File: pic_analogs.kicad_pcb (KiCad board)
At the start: 2 copper layers, 99.1 x 98.4 mm, 242 parts, among them J1 VFWD, J10 USB_B_Mini, J11 term_, J12 term_, J13 term_, J14 term_, J15 term_, J16 term_, J17 term_, J18 term_, J19 term_, J2 IN_RF, J20 term_, J21 term_, J22 term_, J23 term_, J24 term_, J25 term_, J26 term_, J27 term_, J28 term_, J29 term_, J3 OUT_RF, J30 term_, J31 term_, J32 ICD, J33 Micro_SD_Card, J34 Raspberry_Pi_zero_2w, J35 USB_A, J36 OledSpiST1306, J37 OledSpiST7789, J38 ads1115, J39 SI5351, J4 VREV, J40 IN_RF, J41 IN_RF, J42 OledSpiST1306, J43 tp_ft232_, J44 tp_ft232_, J45 tp_ft232_, J46 tp_ft232_, J47 tp_ft232_, J48 tp_ft232_, J49 tp_ft232_, J5 pickit, J50 tp_ft232_, J51 tp_ft232_, J52 USB_B_Mini, J53 F32R-1A7H1-11024, J54 tp_epaper, J56 tp_epaper, J57 tp_epaper, J58 tp_epaper, J59 tp_epaper, Q1 PMOS, SW1 mclr, SW2 rb4, SW3 rb5, SW4 mclr, SW5 ra5, SW6 ra4, SW7 ra5, U2 LM1117DT-3.3, U3 PIC18F4550-IPT, U4 ADS1115IDGS, U5 MRF24J40MA, U6 FT232BM, U7 LM1117DT-3.3, U8 25LCxxx, Y1 Crystal_GND24_Small, Y2 6Mhz

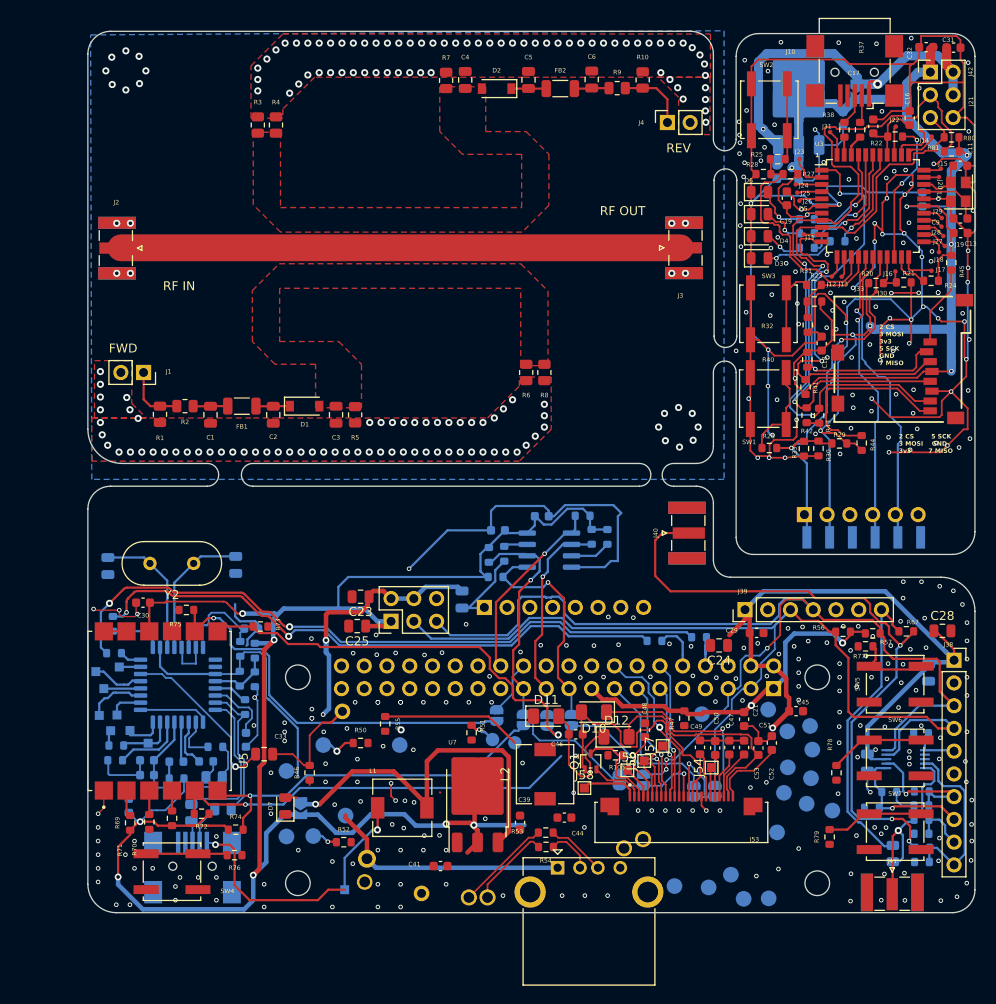
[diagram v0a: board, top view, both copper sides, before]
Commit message: Update
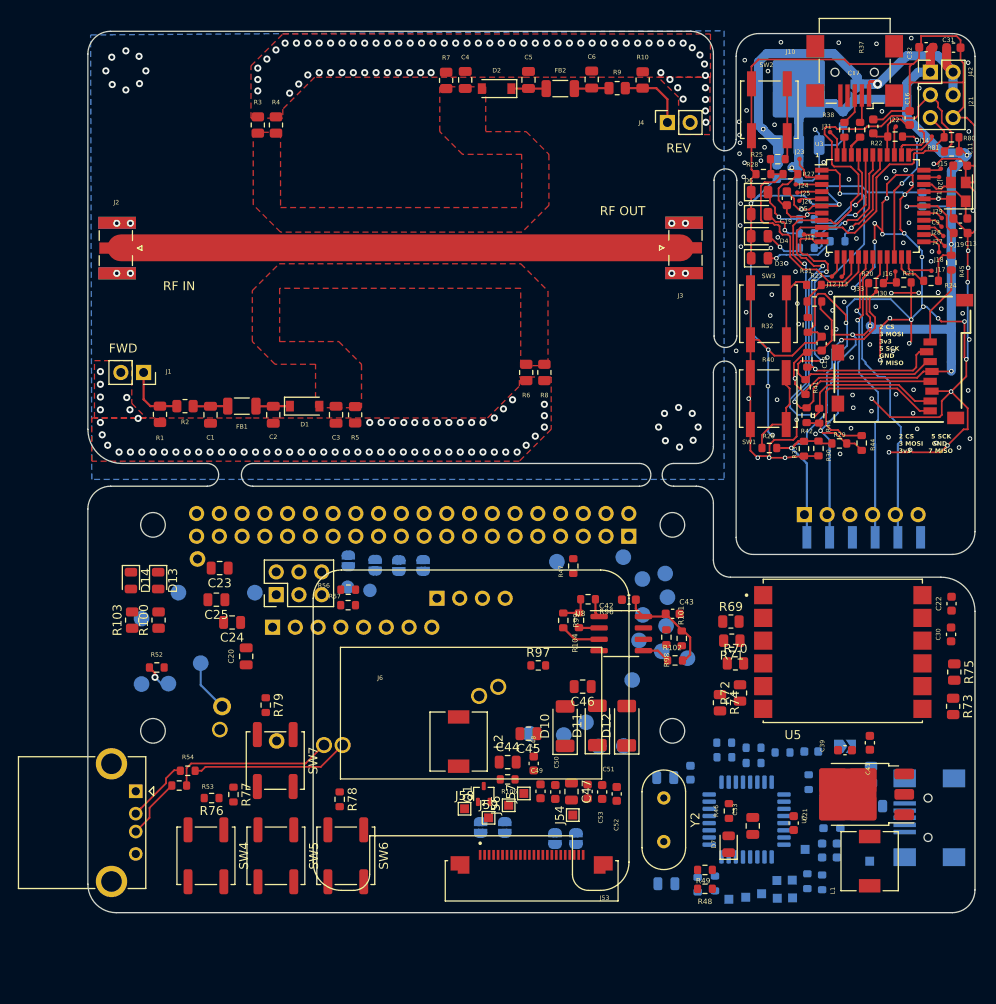
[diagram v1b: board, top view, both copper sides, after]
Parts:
- removed C26, C27, C28: 100nf, Capacitor_SMD:C_0805_2012Metric
- removed C29: 100n, Capacitor_SMD:C_0603_1608Metric
- removed J38: ads1115, Connector_PinSocket_2.54mm:PinSocket_1x10_P2.54mm_Vertical
- removed J39: SI5351, Connector_PinHeader_2.54mm:PinHeader_1x07_P2.54mm_Vertical
- removed J40, J41: IN_RF, Connector_Coaxial:SMA_Samtec_SMA-J-P-X-ST-EM1_EdgeMount
- removed R50, R51, R55: 4K7, Resistor_SMD:R_0603_1608Metric
- removed R58, R60, R62, R64, R66, R67: 10K, Resistor_SMD:R_0603_1608Metric
- removed R59, R61, R63, R65: 1K, Resistor_SMD:R_0603_1608Metric
- removed R68: 10K, Resistor_SMD:R_0805_2012Metric
- removed U4: ADS1115IDGS, Package_SO:TSSOP-10_3x3mm_P0.5mm
- added D13: RX, Diode_SMD:D_0805_2012Metric, F.Cu at (126.6, 140.1)
- added D14: RX, Diode_SMD:D_0805_2012Metric, F.Cu at (123.6, 140.1)
- added J6: oled128x64, kiC:SSD1306_No_Mounting_whitout_Holes, F.Cu at (152.6, 142.1)
- added R100: 2k2, Resistor_SMD:R_0805_2012Metric, F.Cu at (126.6, 144.5)
- added R103: 2k2, Resistor_SMD:R_0805_2012Metric, F.Cu at (123.7, 144.5)
- added R97: 2k2, Resistor_SMD:R_0603_1608Metric, F.Cu at (169.0, 149.6)
- C20, C22, C42, C43, R101, R102, R104, R48, R49, R96, R98, R99, U8: moved to F.Cu
- C44, C45, C46, C47: footprint Capacitor_SMD:C_0603_1608Metric -> Capacitor_SMD:C_0805_2012Metric
- D10, D11, D12: footprint Diode_SMD:D_1206_3216Metric -> Diode_SMD:D_SOD-128
- R69, R70, R71, R72, R73, R74, R75: footprint Resistor_SMD:R_0603_1608Metric -> Resistor_SMD:R_0805_2012Metric
- moved C22 94.6 mm to (215.2, 142.7)
- moved C30 90.3 mm to (215.1, 146.1), turned to 90 degrees
- moved R75 86.0 mm to (215.5, 150.3), turned to -90 degrees
- moved J52 82.3 mm to (212.6, 166.6), turned to -90 degrees
- moved R82 80.1 mm to (200.7, 173.8), turned to 90 degrees
- moved R83 78.6 mm to (199.1, 173.6), turned to -90 degrees
- moved J44 78.4 mm to (195.7, 175.6), turned to -90 degrees
- moved J50 78.4 mm to (197.4, 175.5), turned to 90 degrees
- moved R73 77.9 mm to (215.4, 154.1), turned to -90 degrees
- moved C35 77.5 mm to (202.4, 170.2), turned to 90 degrees
- moved J45 76.9 mm to (194.0, 175.0), turned to -90 degrees
- moved J49 76.8 mm to (192.2, 175.4), turned to -90 degrees
- moved U5 76.6 mm to (203.0, 147.9), turned to 0 degrees
- moved R94 76.3 mm to (206.6, 165.3), turned to 0 degrees
- moved C34 76.1 mm to (200.7, 170.2), turned to 90 degrees
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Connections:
- J34 pad 3: SDA_OLED_RPI -> SDA_RPI
- J34 pad 5: SCL_OLED_RPI -> SCL_RPI
- J34 pad 56: /magnetics/mcu_pic/rpi/TV -> Net-(J34-TV)
- J34 pad 67: Net-(J34-CORE) -> /magnetics/mcu_pic/rpi/CORE_RPI
- J34 pad 71: Net-(J34-WL_ON) -> unconnected-(J34-WL_ON-Pad71)
- J34 pad 72: Net-(J34-BT_ON) -> unconnected-(J34-BT_ON-Pad72)
- J37 pad 3: /magnetics/mcu_pic/rpi/display_oled/SCKL_SST -> GPIO26
- J37 pad 4: /magnetics/mcu_pic/rpi/display_oled/SDIN -> GPIO19
- JP4 pad 1: SCL_OLED_RPI -> SCL_RPI
- JP6 pad 1: SDA_OLED_RPI -> SDA_RPI
- R92 pad 2: USB_D- -> USB_D+
- U6 pad 7: USB_D- -> USB_D+
- U6 pad 8: USB_D+ -> USB_D-
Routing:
- net +3V3: track 265.9 -> 15.2 mm, vias 9 -> 0
- net +5V: track 131.6 -> 5.81 mm, vias 3 -> 0
- net SCL_OLED_RPI: track 117.4 -> 0.00 mm, vias 3 -> 0
- net GND: track 488.4 -> 371.3 mm, vias 480 -> 274
- net SDA_OLED_RPI: track 107.7 -> 0.00 mm
- net TX_RPI: track 75.9 -> 0.00 mm, vias 2 -> 0
- net V+_USB: track 74.9 -> 0.00 mm, vias 1 -> 0
- net MEASURE_ADDR0: track 72.6 -> 0.00 mm, vias 3 -> 0
- net RX_RPI: track 66.1 -> 0.00 mm, vias 2 -> 0
- net /magnetics/mcu_pic/rpi/mrf24j40/MISO_mrf24j40: track 47.8 -> 0.00 mm, vias 1 -> 0
- net /magnetics/mcu_pic/rpi/mrf24j40/MOSI_mrf24j40: track 46.4 -> 0.00 mm, vias 1 -> 0
- net /magnetics/mcu_pic/rpi/mrf24j40/CE0_mrf24j40: track 45.3 -> 0.00 mm, vias 1 -> 0
- net /magnetics/mcu_pic/rpi/mrf24j40/SCLK_mrf24j40: track 41.8 -> 0.00 mm, vias 1 -> 0
- net SCLK: track 40.3 -> 0.00 mm, vias 1 -> 0
- net MOSI: track 42.4 -> 3.16 mm, vias 1 -> 0
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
